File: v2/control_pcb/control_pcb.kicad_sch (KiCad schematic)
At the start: 24 parts, among them J1 Raspberry_Pi_2_3, J10 8P8C_Shielded, J11 Screw_Terminal_01x02, J12 Screw_Terminal_01x02, J13 Screw_Terminal_01x02, J2 8P8C_Shielded, J6 Screw_Terminal_01x02, J7 Screw_Terminal_01x02, J8 Screw_Terminal_01x08, J9 Screw_Terminal_01x08, U3 Raspberry_Pi_Pico_2, U4 TCA9509DGKR, U5 TXU0304PWR

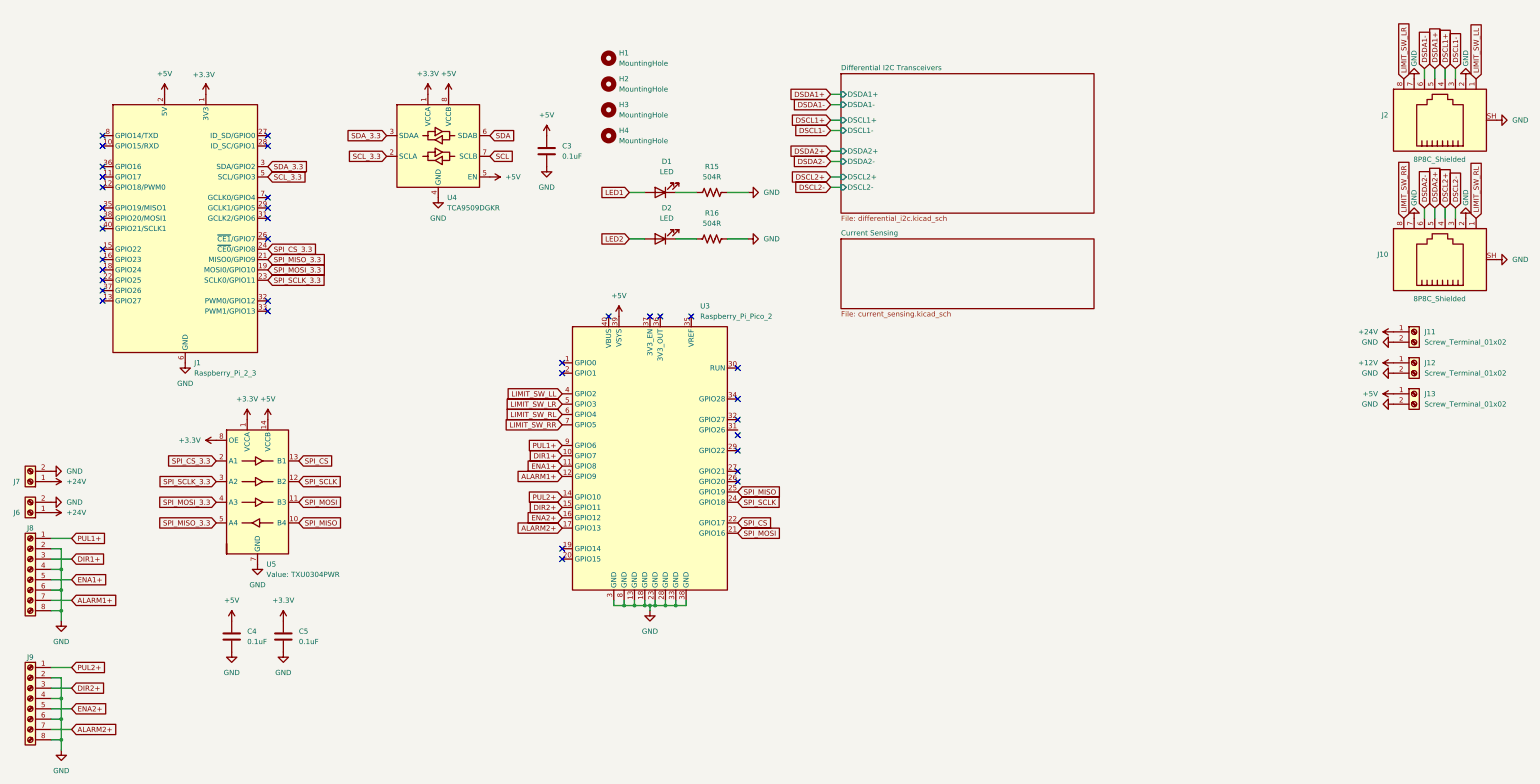
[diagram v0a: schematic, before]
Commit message: Preliminary V2 schematics
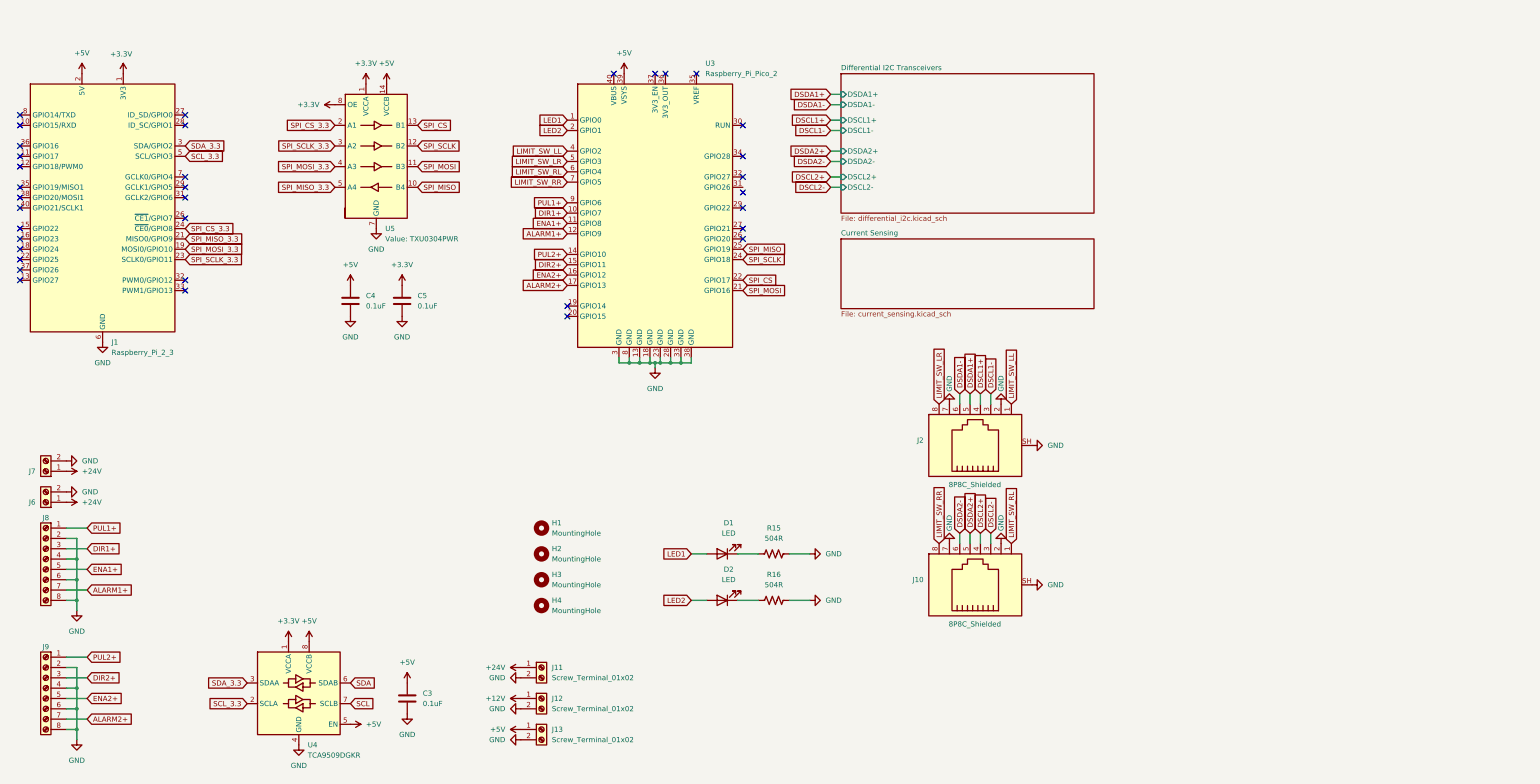
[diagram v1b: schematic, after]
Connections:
- net LED1: now also U3.1 (GPIO0)
- net LED2: now also U3.2 (GPIO1)
- no-connect marks 37 -> 35
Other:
- moved on the sheet: C3, C4, C5, D1, D2, H1, H2, H3, H4, J1, J10, J11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

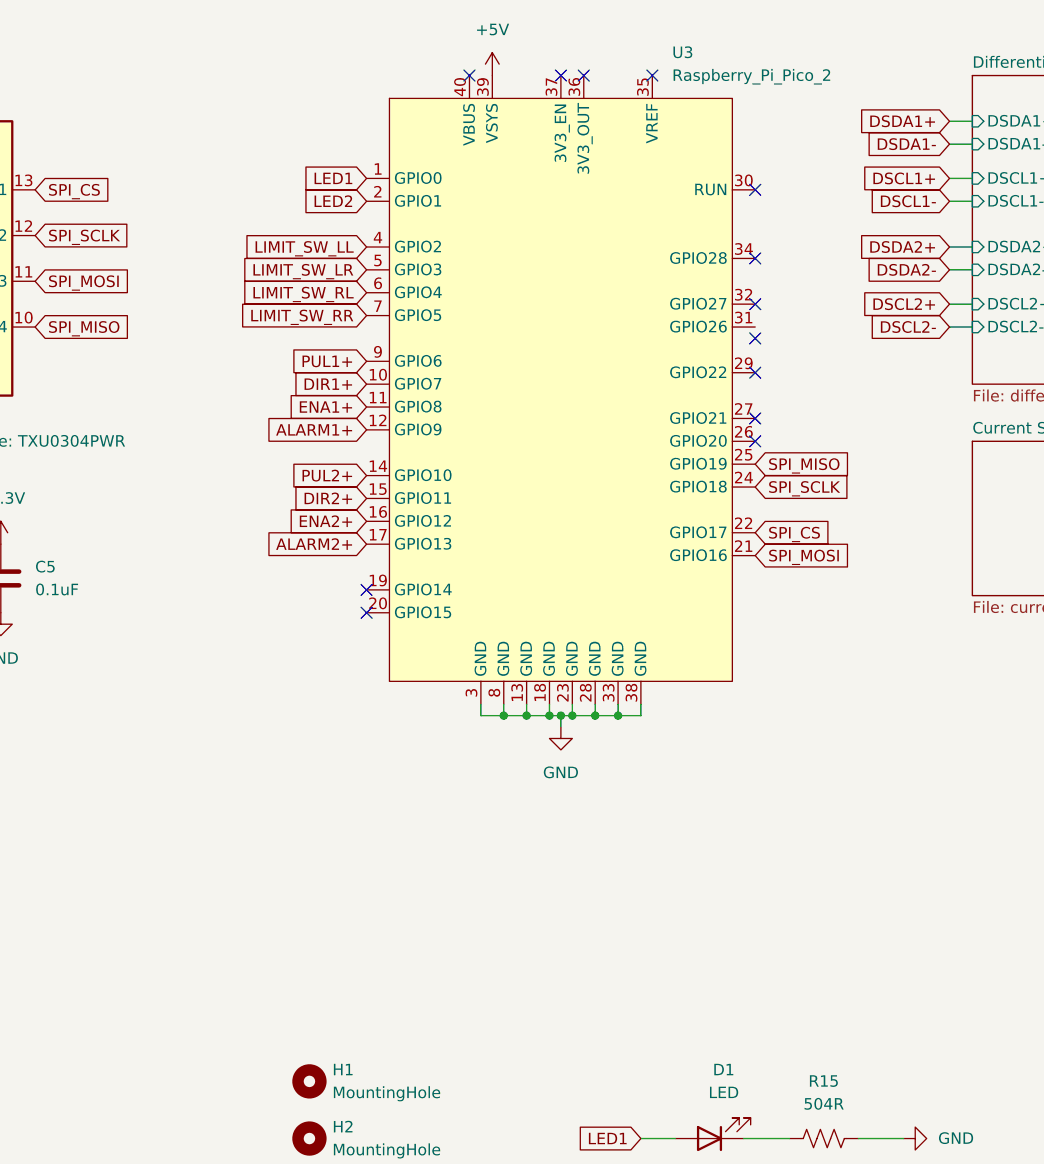
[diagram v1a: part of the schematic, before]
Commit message: Doing stuff
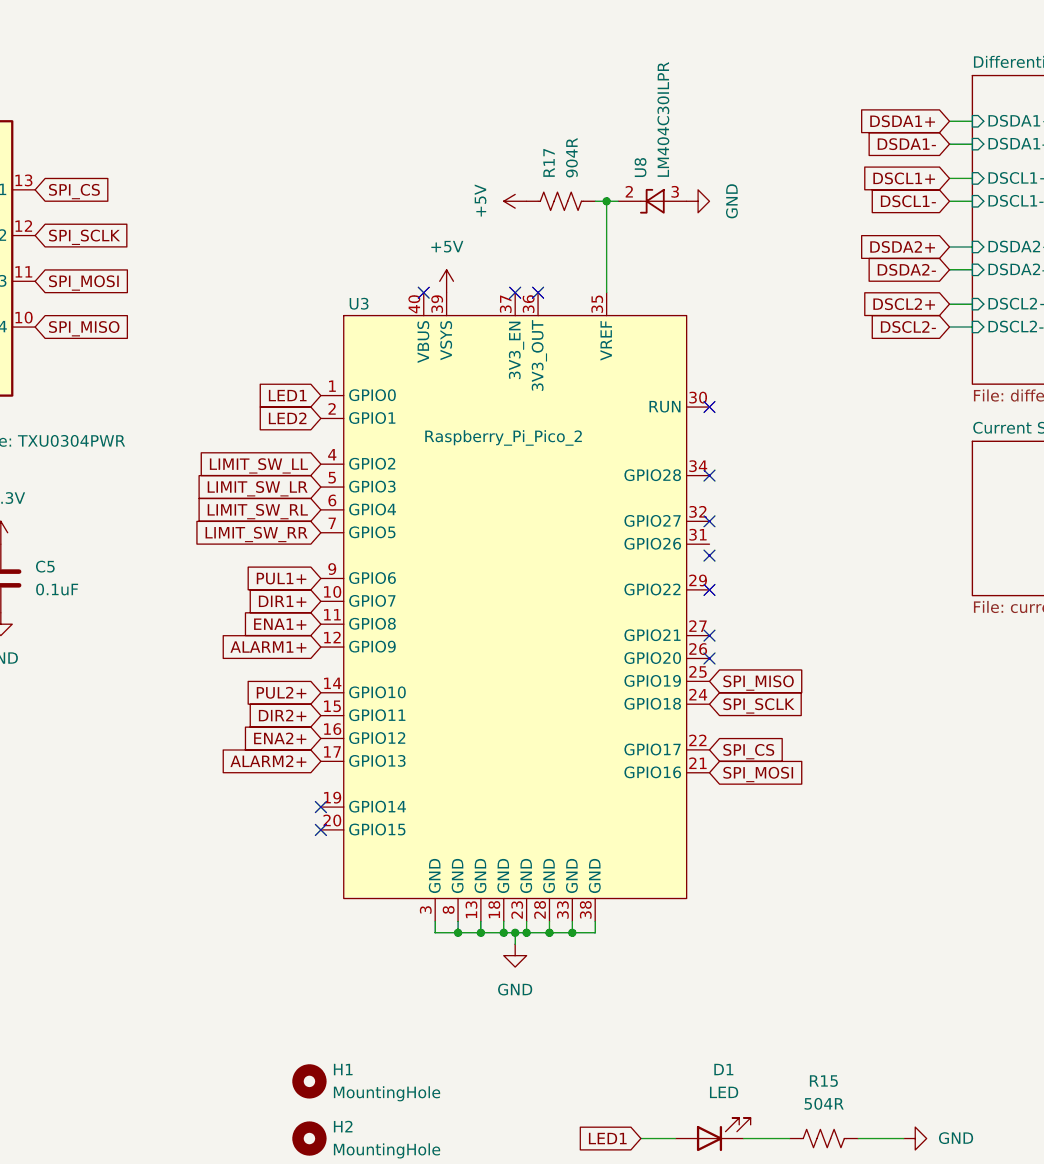
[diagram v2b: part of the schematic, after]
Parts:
- added R17: 904R, Resistor_THT:R_Axial_DIN0207_L6.3mm_D2.5mm_P10.16mm_Horizontal, symbol Device:R_US
- added U8: LM404C30ILPR, Package_TO_SOT_THT:TO-92_Inline, symbol Reference_Voltage:LM4040LP-4.1
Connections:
- net +5V: now also R17.1
- net GND: now also U8.3 (A)
- net at U3.35 (VREF): now also R17.2, U8.2 (K)
- no-connect marks 35 -> 34
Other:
- moved on the sheet: U3

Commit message: Doing some things
Crossing some ts and dotting some is. Making v3 of the BOM.
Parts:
- U3: Digikey (none) -> https://www.digikey.ca/en/products/detail/raspberry-pi/SC16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
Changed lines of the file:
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@@
 		(on_board yes)
 		(dnp no)
-		(fields_autoplaced yes)
 		(property "Reference" "#PWR038"
 			(at 81.28 165.1 0)
@@
 		)
 		(property "Description" ""
+			(at 144.78 57.15 0)
+			(effects
+				(font
+					(size 1.27 1.27)
+				)
+				(hide yes)
+			)
+		)
+		(property "Digikey" "https://www.digikey.ca/en/products/detail/raspberry-pi/SC1631/24627136"
 			(at 144.78 57.15 0)
 			(effects
@@
 		(on_board yes)
 		(dnp no)
-		(fields_autoplaced yes)
 		(property "Reference" "#PWR039"
 			(at 86.36 165.1 0)
